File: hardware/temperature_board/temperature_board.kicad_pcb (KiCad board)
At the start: 2 copper layers, 91 x 21 mm, 13 parts, among them J1 RJ45, U1 TSIC50XF, U2 ST485, m3_loch VAL**

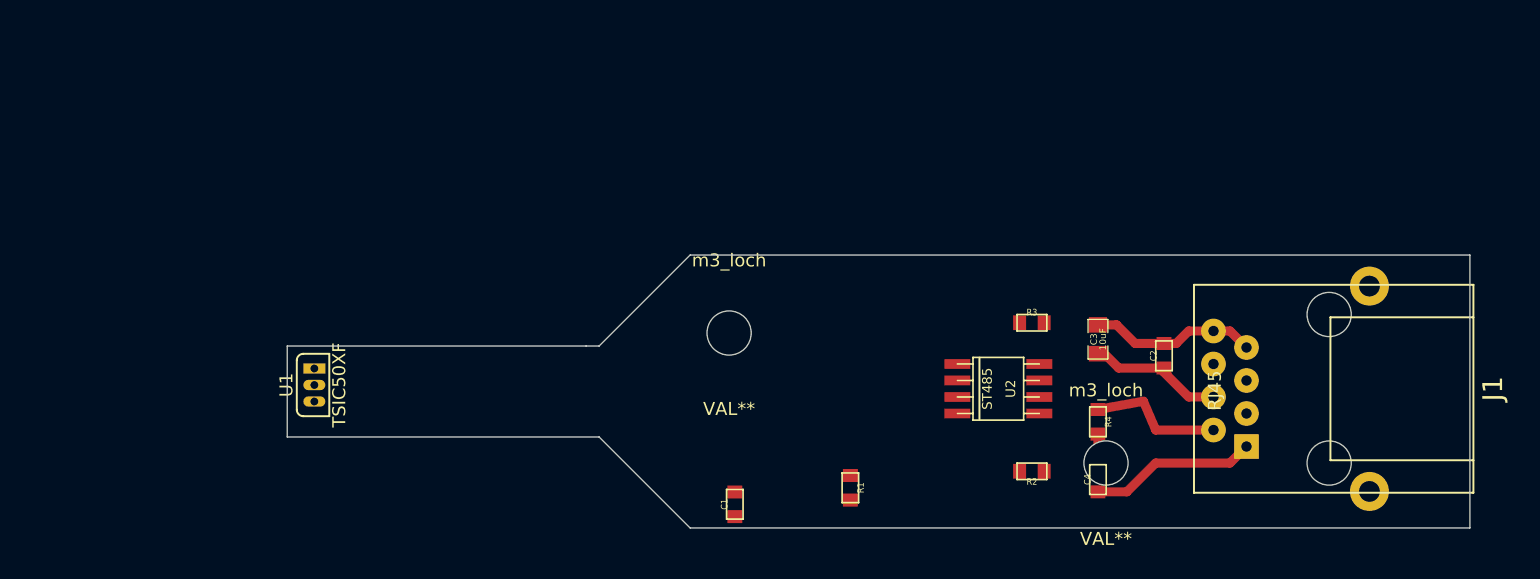
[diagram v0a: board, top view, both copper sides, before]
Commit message: temperature board pcb finished
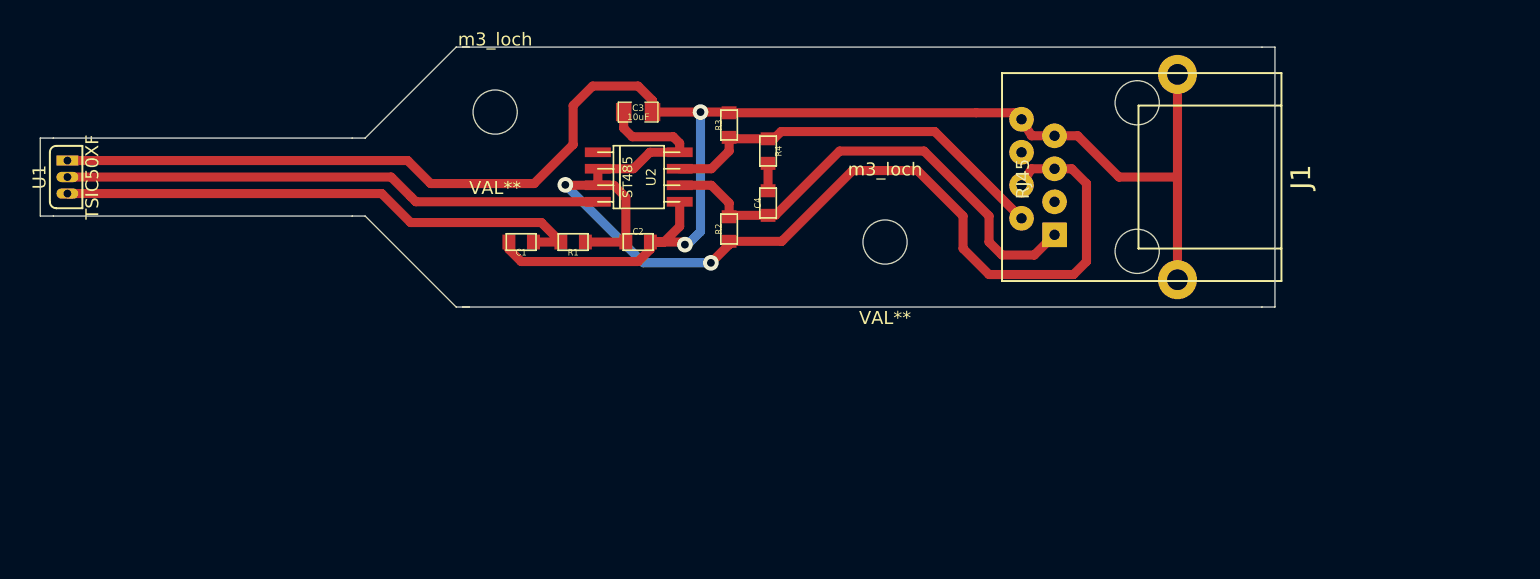
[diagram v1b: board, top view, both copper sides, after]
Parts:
- moved C2 41.4 mm to (211.0, 150.0), turned to 0 degrees
- moved C3 39.5 mm to (211.0, 140.0), turned to 0 degrees
- moved C4 33.1 mm to (221.0, 147.0)
- moved R4 32.8 mm to (221.0, 143.0)
- moved U2 32.1 mm to (213.0, 145.0)
- moved R2 29.8 mm to (218.0, 149.0), turned to 90 degrees
- moved R1 28.5 mm to (206.0, 150.0), turned to 180 degrees
- moved R3 27.8 mm to (218.0, 141.0), turned to 90 degrees
- moved C1 26.0 mm to (202.0, 150.0), turned to 180 degrees
- moved U1 24.8 mm to (169.0, 145.0)
- moved m3_loch 24.8 mm to (200.0, 140.0)
- moved m3_loch 24.0 mm to (230.0, 150.0)
- moved J1 22.0 mm to (240.5, 145.0)
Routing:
- net GND: track 12.9 -> 142.1 mm, vias 0 -> 2
- net VCC: track 10.5 -> 89.5 mm, vias 0 -> 2
- net N-0000010: track 0.00 -> 41.6 mm
- net N-000007: track 0.00 -> 41.6 mm
- net /za: track 12.9 -> 37.7 mm
- net /zb: track 10.4 -> 31.0 mm
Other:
- board size 91 x 21 mm -> 95 x 20 mm
